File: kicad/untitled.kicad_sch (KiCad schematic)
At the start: 2 parts, among them U1 TLC5916IN

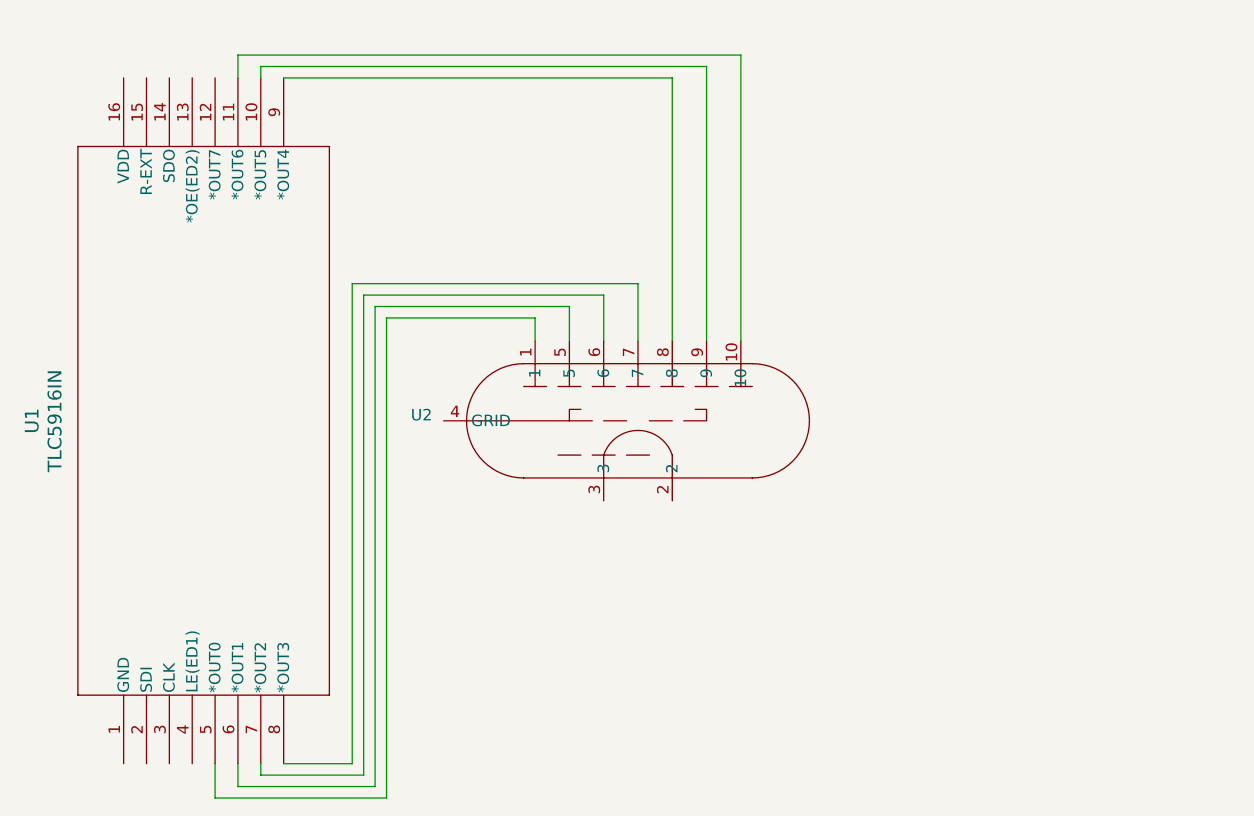
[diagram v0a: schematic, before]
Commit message: added controller
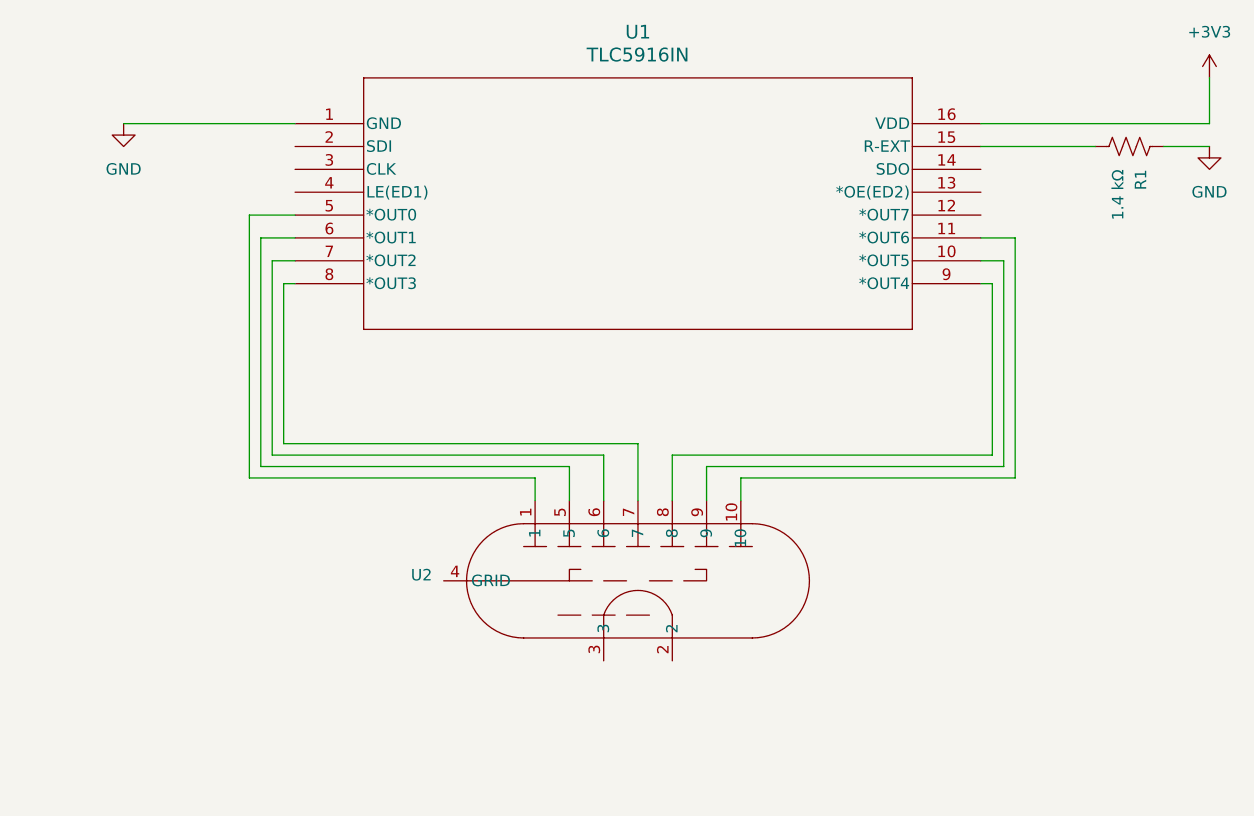
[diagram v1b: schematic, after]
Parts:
- added R1: 1.4 kΩ, symbol Device:R_US
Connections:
- net GND: now reaches U1.1 (GND)
- net GND: now also R1.1
- net at U1.15 (R-EXT): now also R1.2
- net +3V3: now reaches U1.16 (VDD)
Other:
- moved on the sheet: U1, U2
